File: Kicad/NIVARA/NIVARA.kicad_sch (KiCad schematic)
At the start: 1 part, among them J1 Screw_Terminal_01x02

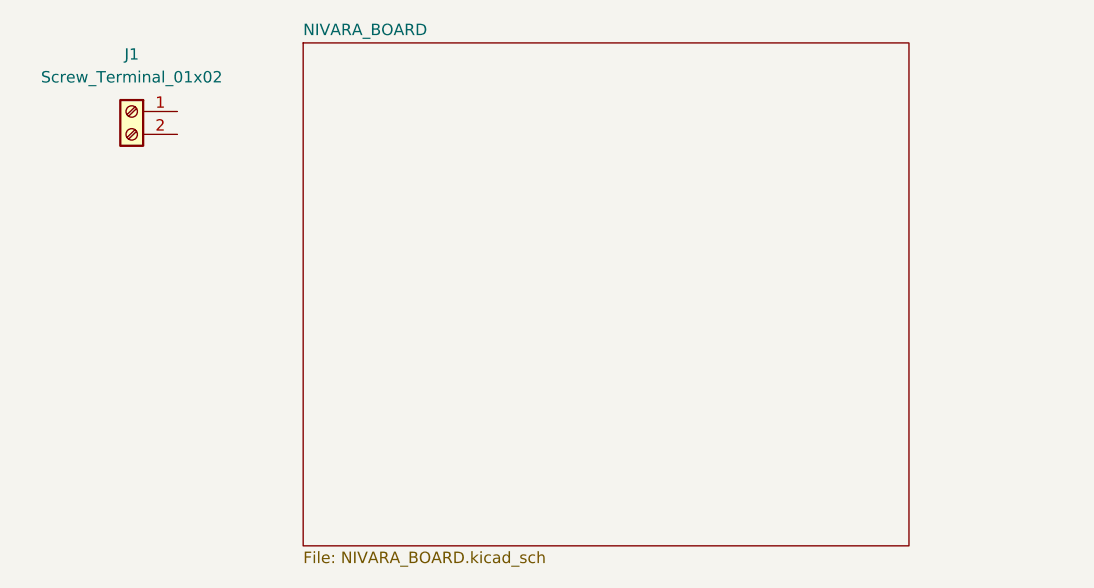
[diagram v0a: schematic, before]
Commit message: Initial Capture Finished
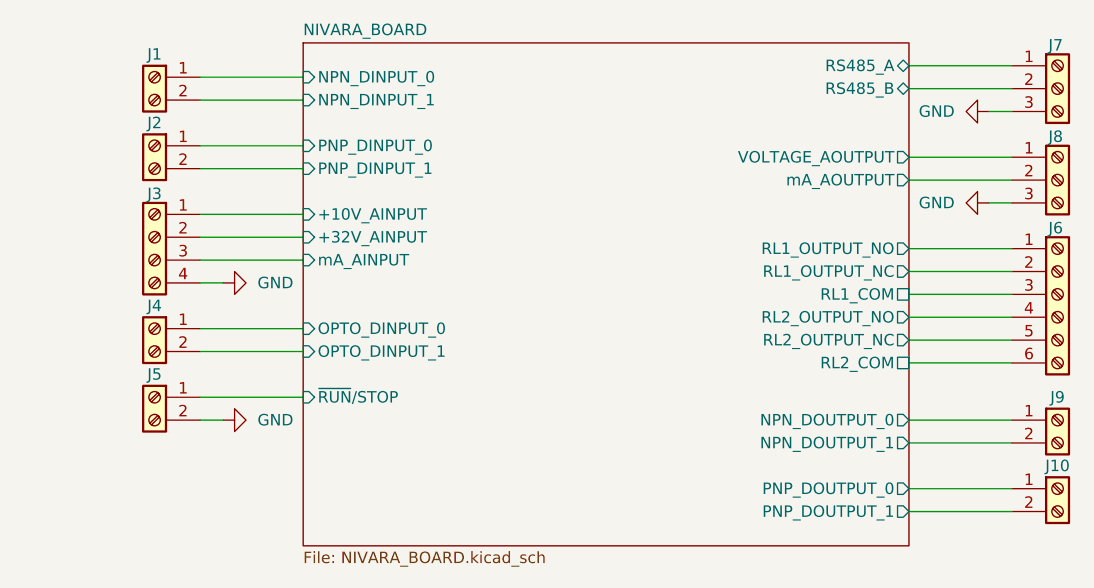
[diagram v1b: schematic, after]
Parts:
- added J10, J2, J4, J5, J9: Screw_Terminal_01x02, symbol Connector:Screw_Terminal_01x02
- added J3: Screw_Terminal_01x04, symbol Connector:Screw_Terminal_01x04
- added J6: Screw_Terminal_01x06, symbol Connector:Screw_Terminal_01x06
- added J7, J8: Screw_Terminal_01x03, symbol Connector:Screw_Terminal_01x03
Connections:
- net NIVARA_BOARD/NPN_DINPUT_0: now reaches J1.1 (Pin_1)
- net NIVARA_BOARD/NPN_DINPUT_1: now reaches J1.2 (Pin_2)
- new net GND: J3.4 (Pin_4), J5.2 (Pin_2), J7.3 (Pin_3), J8.3 (Pin_3)
- new net NIVARA_BOARD/+10V_AINPUT: J3.1 (Pin_1)
- new net NIVARA_BOARD/+32V_AINPUT: J3.2 (Pin_2)
- new net NIVARA_BOARD/NPN_DOUTPUT_0: J9.1 (Pin_1)
- new net NIVARA_BOARD/NPN_DOUTPUT_1: J9.2 (Pin_2)
- new net NIVARA_BOARD/OPTO_DINPUT_0: J4.1 (Pin_1)
- new net NIVARA_BOARD/OPTO_DINPUT_1: J4.2 (Pin_2)
- new net NIVARA_BOARD/PNP_DINPUT_0: J2.1 (Pin_1)
- new net NIVARA_BOARD/PNP_DINPUT_1: J2.2 (Pin_2)
- new net NIVARA_BOARD/PNP_DOUTPUT_0: J10.1 (Pin_1)
- new net NIVARA_BOARD/PNP_DOUTPUT_1: J10.2 (Pin_2)
- new net NIVARA_BOARD/RL1_COM: J6.3 (Pin_3)
- new net NIVARA_BOARD/RL1_OUTPUT_NC: J6.2 (Pin_2)
- new net NIVARA_BOARD/RL1_OUTPUT_NO: J6.1 (Pin_1)
- new net NIVARA_BOARD/RL2_COM: J6.6 (Pin_6)
- new net NIVARA_BOARD/RL2_OUTPUT_NC: J6.5 (Pin_5)
- new net NIVARA_BOARD/RL2_OUTPUT_NO: J6.4 (Pin_4)
- new net NIVARA_BOARD/RS485_A: J7.1 (Pin_1)
- new net NIVARA_BOARD/RS485_B: J7.2 (Pin_2)
- new net NIVARA_BOARD/VOLTAGE_AOUTPUT: J8.1 (Pin_1)
- new net NIVARA_BOARD/mA_AINPUT: J3.3 (Pin_3)
- new net NIVARA_BOARD/mA_AOUTPUT: J8.2 (Pin_2)
- new net NIVARA_BOARD/~{RUN}/STOP: J5.1 (Pin_1)
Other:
- sheet NIVARA_BOARD ports: added +10V_AINPUT, +32V_AINPUT, NPN_DINPUT_0, NPN_DINPUT_1, NPN_DOUTPUT_0, NPN_DOUTPUT_1, OPTO_DINPUT_0, OPTO_DINPUT_1, PNP_DINPUT_0, PNP_DINPUT_1, PNP_DOUTPUT_0, PNP_DOUTPUT_1, RL1_COM, RL1_OUTPUT_NC, RL1_OUTPUT_NO, RL2_COM, RL2_OUTPUT_NC, RL2_OUTPUT_NO, RS485_A, RS485_B, VOLTAGE_AOUTPUT, mA_AINPUT, mA_AOUTPUT, ~{RUN}/STOP; removed none
- moved on the sheet: J1
